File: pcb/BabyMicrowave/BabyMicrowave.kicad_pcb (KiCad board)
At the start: 2 copper layers, 67.8 x 18.3 mm, 12 parts, among them J1 Power, J2 Timer, SW1 Power Switch, SW2 Door Switch, U1 ATtiny13A-P

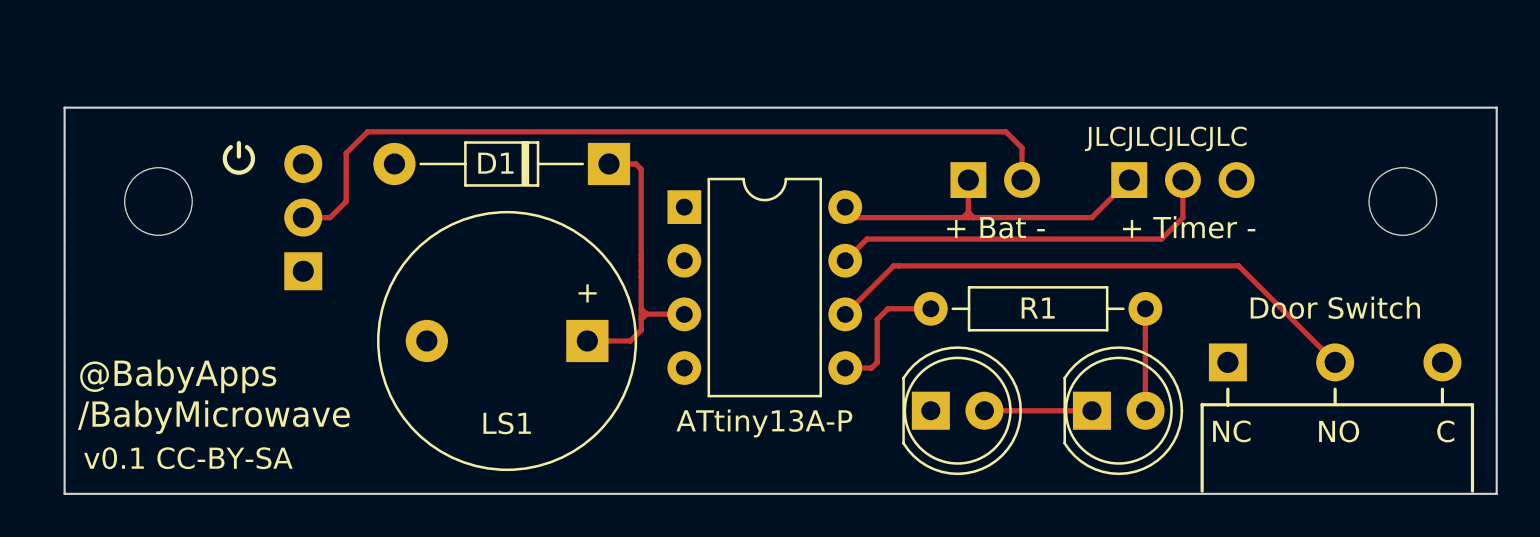
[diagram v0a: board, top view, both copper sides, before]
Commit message: WIP - relayout.
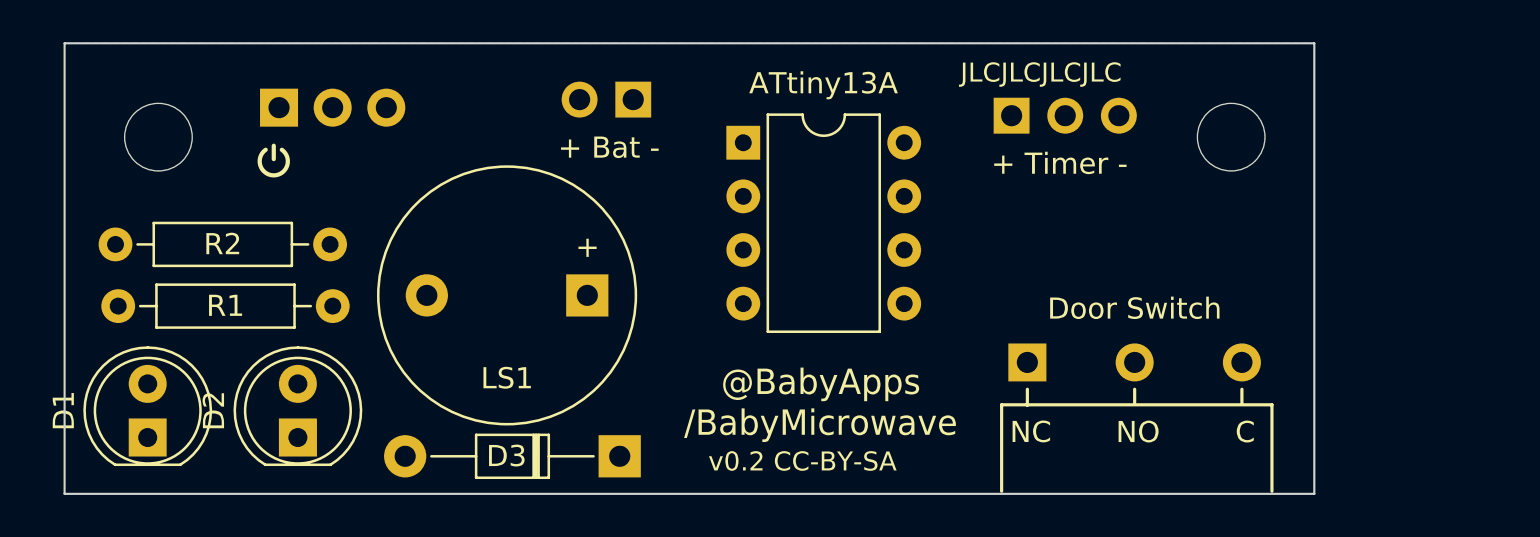
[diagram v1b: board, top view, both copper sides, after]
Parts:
- removed the D3 at (144.3, 58.2)
- added D1: LED, LED_THT:LED_D5.0mm, F.Cu at (107.2, 59.4)
- added R2: R, Resistor_THT:R_Axial_DIN0207_L6.3mm_D2.5mm_P10.16mm_Horizontal, F.Cu at (115.8, 50.3)
- U1: value ATtiny13A-P -> ATtiny13A
- moved D2 37.6 mm to (114.3, 59.4), turned to 90 degrees
- moved R1 28.3 mm to (116.0, 53.2), turned to 180 degrees
- moved J1 16.3 mm to (130.2, 43.4), turned to -90 degrees
- moved D3 13.9 mm to (129.5, 60.3)
- moved SW2 9.49 mm to (153.9, 55.9)
- moved REF** 8.68 mm to (158.5, 45.2)
- moved J2 6.35 mm to (148.1, 44.2)
- moved SW1 5.39 mm to (115.9, 43.8), turned to 0 degrees
- moved U1 4.13 mm to (135.4, 45.5)
- moved REF** 3.05 mm to (107.7, 45.2)
- moved LS1 2.16 mm to (128.0, 52.7)
- renumbered D1 to D3
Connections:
- D2 pad 1: Net-(D2-Pad1) -> GND
- R1 pad 2: Net-(D2-Pad2) -> Net-(D1-Pad2)
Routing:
- net Net-(J1-Pad2): track 38.9 -> 0.00 mm
- net Net-(SW2-Pad2): track 26.0 -> 0.00 mm
- net Net-(J2-Pad2): track 18.6 -> 0.00 mm
- net Net-(J1-Pad1): track 16.9 -> 0.00 mm
- net Net-(D3-Pad1): track 14.5 -> 0.00 mm
- net Net-(R1-Pad1): track 6.41 -> 0.00 mm
- net Net-(D2-Pad1): track 5.09 -> 0.00 mm
- net Net-(D2-Pad2): track 4.83 -> 0.00 mm
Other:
- board size 67.8 x 18.3 mm -> 59.2 x 21.3 mm
- board text added: "v0.2 CC-BY-SA"
- board text removed: "v0.1 CC-BY-SA"
